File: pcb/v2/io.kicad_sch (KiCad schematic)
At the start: 63 parts, among them J10 Conn_01x05, J14 Conn_01x04, Q3 PMOS, Q4 NPN, U7 TCKE812, U8 CH334R, U9 STI9287, Y1 12M

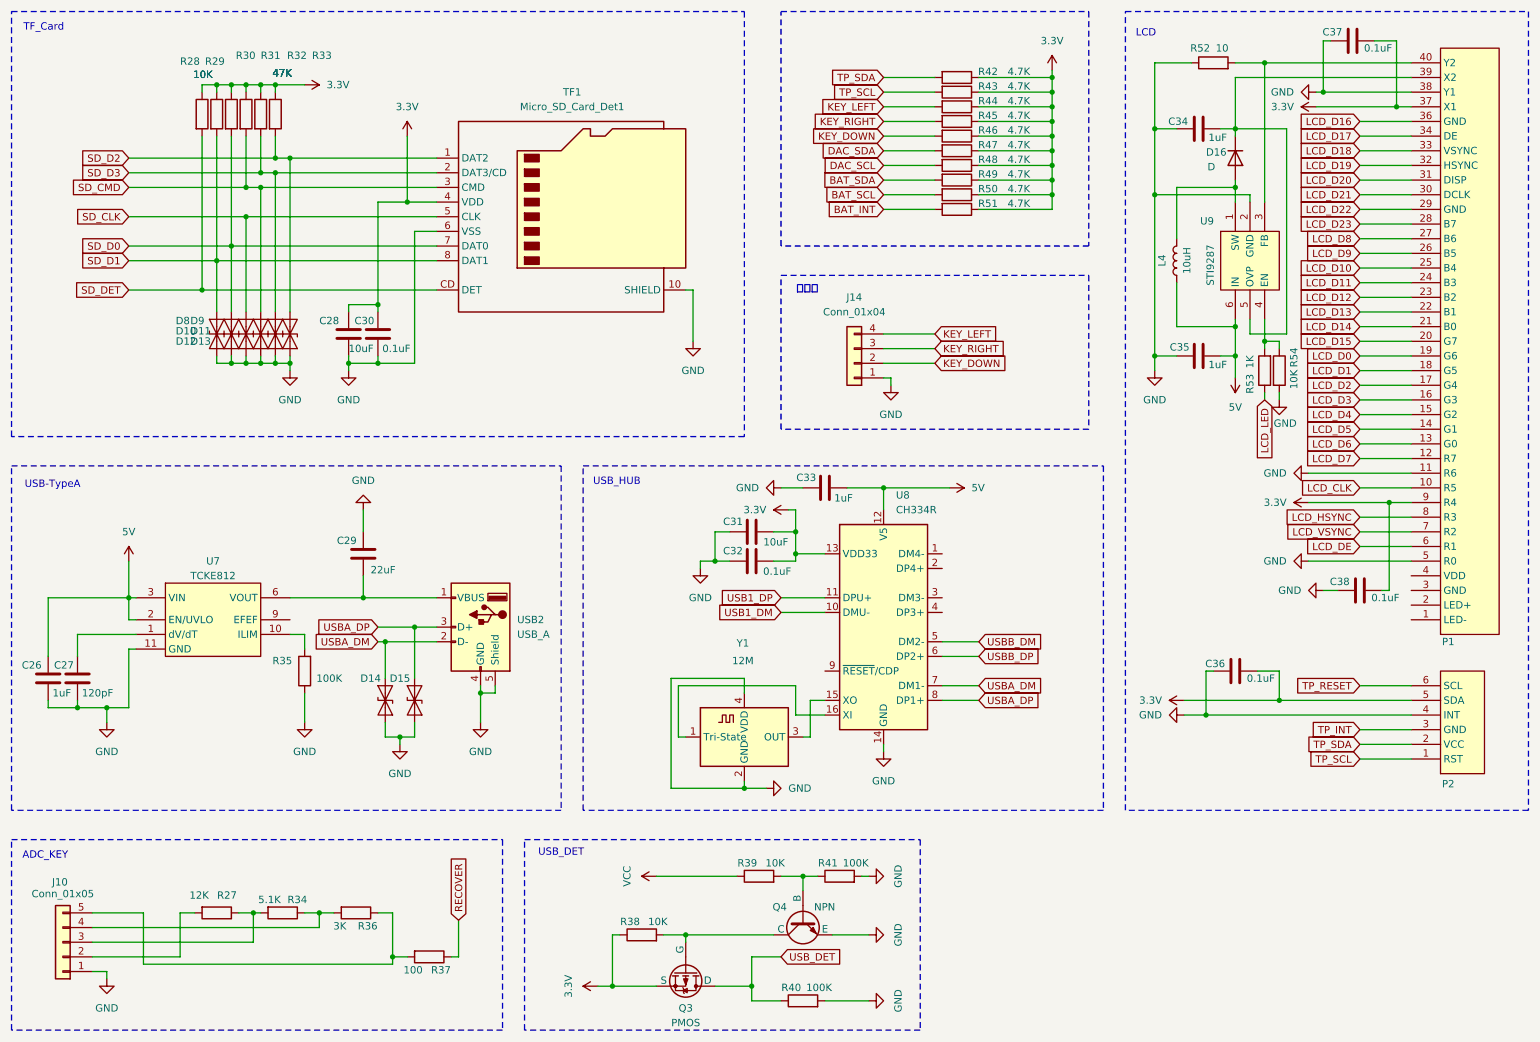
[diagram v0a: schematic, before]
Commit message: up fix lcd pcb
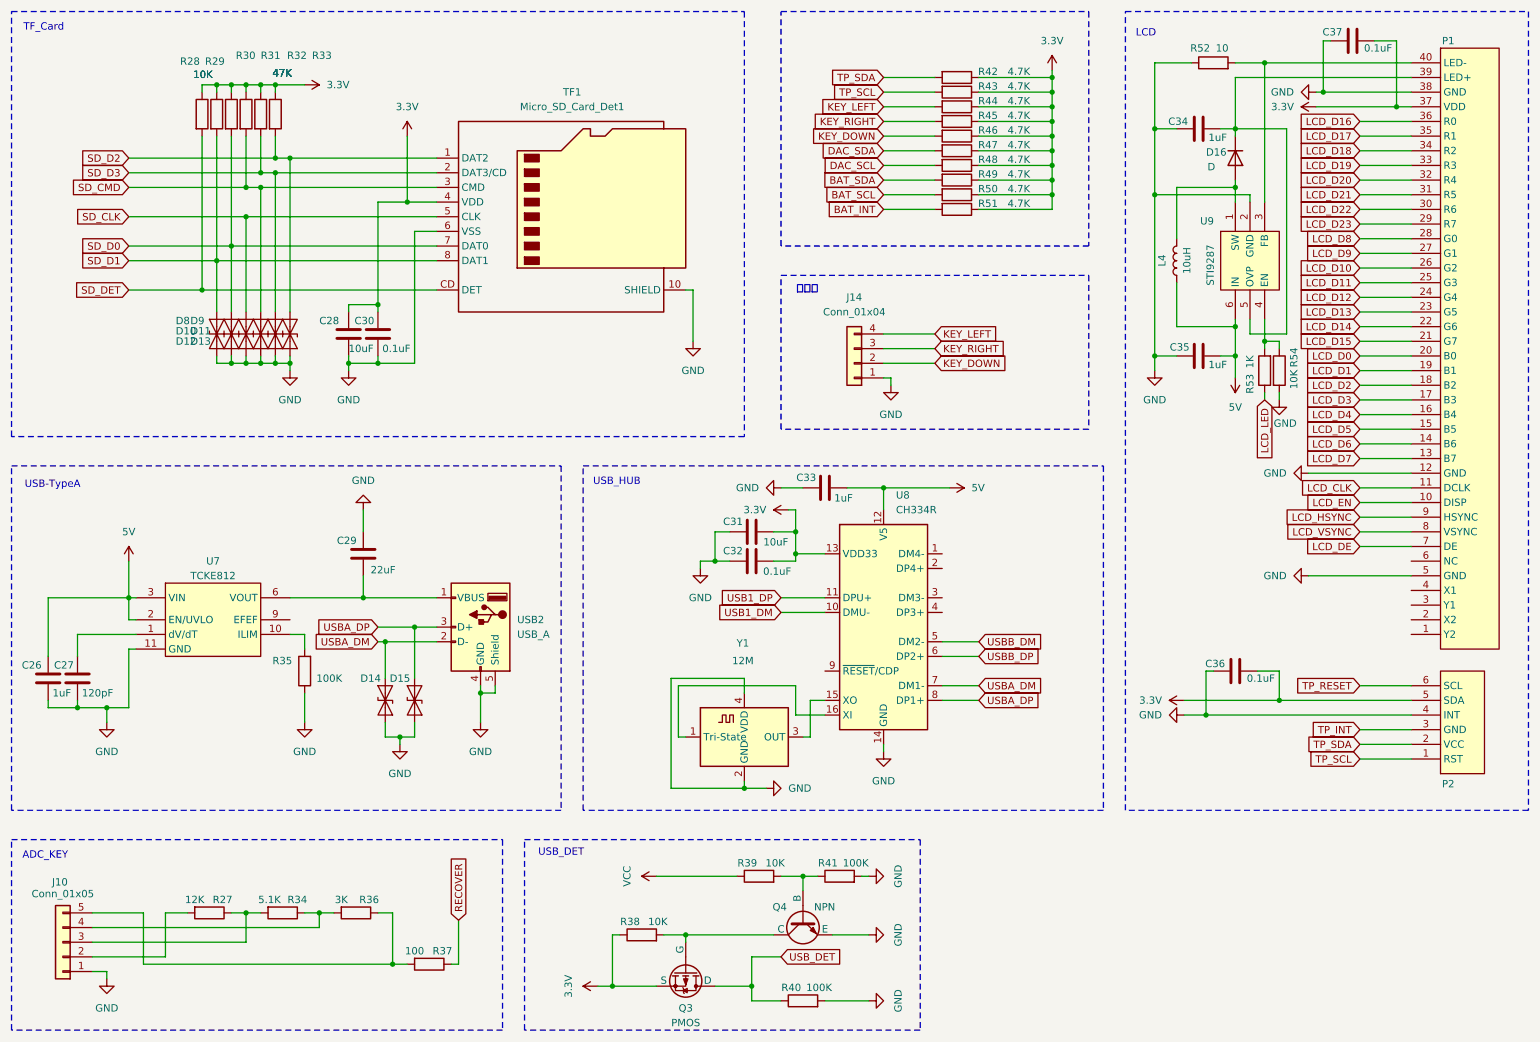
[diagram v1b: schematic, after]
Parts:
- removed C38: 0.1uF, Capacitor_SMD:C_0402_1005Metric_Pad0.74x0.62mm_HandSolder, symbol Device:C
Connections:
- net 3.3V: no longer P1.9 (R4)
- net GND: now also P1.12 (GND); no longer P1.11 (R6)
- net LCD_CLK: now also P1.11 (DCLK); no longer P1.10 (R5)
- net LCD_D0: now also P1.20 (B0); no longer P1.19 (G6)
- net LCD_D1: now also P1.19 (B1); no longer P1.18 (G5)
- net LCD_D10: now also P1.26 (G2); no longer P1.25 (B4)
- net LCD_D11: now also P1.25 (G3); no longer P1.24 (B3)
- net LCD_D12: now also P1.24 (G4); no longer P1.23 (B2)
- net LCD_D13: now also P1.23 (G5); no longer P1.22 (B1)
- net LCD_D14: now also P1.22 (G6); no longer P1.21 (B0)
- net LCD_D15: now also P1.21 (G7); no longer P1.20 (G7)
- net LCD_D17: now also P1.35 (R1); no longer P1.34 (DE)
- net LCD_D18: now also P1.34 (R2); no longer P1.33 (VSYNC)
- net LCD_D19: now also P1.33 (R3); no longer P1.32 (HSYNC)
- net LCD_D2: now also P1.18 (B2); no longer P1.17 (G4)
- net LCD_D20: now also P1.32 (R4); no longer P1.31 (DISP)
- net LCD_D21: now also P1.31 (R5); no longer P1.30 (DCLK)
- net LCD_D22: now also P1.30 (R6); no longer P1.29 (GND)
- net LCD_D23: now also P1.29 (R7); no longer P1.28 (B7)
- net LCD_D3: now also P1.17 (B3); no longer P1.16 (G3)
- net LCD_D4: now also P1.16 (B4); no longer P1.15 (G2)
- net LCD_D5: now also P1.15 (B5); no longer P1.14 (G1)
- net LCD_D6: now also P1.14 (B6); no longer P1.13 (G0)
- net LCD_D7: now also P1.13 (B7); no longer P1.12 (R7)
- net LCD_D8: now also P1.28 (G0); no longer P1.27 (B6)
- net LCD_D9: now also P1.27 (G1); no longer P1.26 (B5)
- net LCD_DE: now also P1.7 (DE); no longer P1.6 (R1)
- net LCD_HSYNC: now also P1.9 (HSYNC); no longer P1.8 (R3)
- net LCD_VSYNC: now also P1.8 (VSYNC); no longer P1.7 (R2)
- new net LCD_EN: P1.10 (DISP)
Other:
- moved on the sheet: R27, R37
